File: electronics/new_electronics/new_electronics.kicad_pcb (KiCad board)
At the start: 2 copper layers, 165.1 x 101.6 mm, 48 parts, among them J1 PinHeader_1x03_P2.54mm_Vertic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, K1 Relay_SPDT_Omron-G5Q-1, K2 Relay_SPDT_Omron-G5Q-1, K3 Relay_SPDT_Omron-G5Q-1, K4 Relay_SPDT_Omron-G5Q-1, Q1 TO-92_Inline, Q2 TO-92_Inline, Q3 TO-92_Inline, Q4 TO-92_Inline, Q5 TO-92_Inline, Q6 TO-92_Inline, Q7 TO-92_Inline, Q8 TO-92_Inline, U1 metro_mini, U2 mpu6050

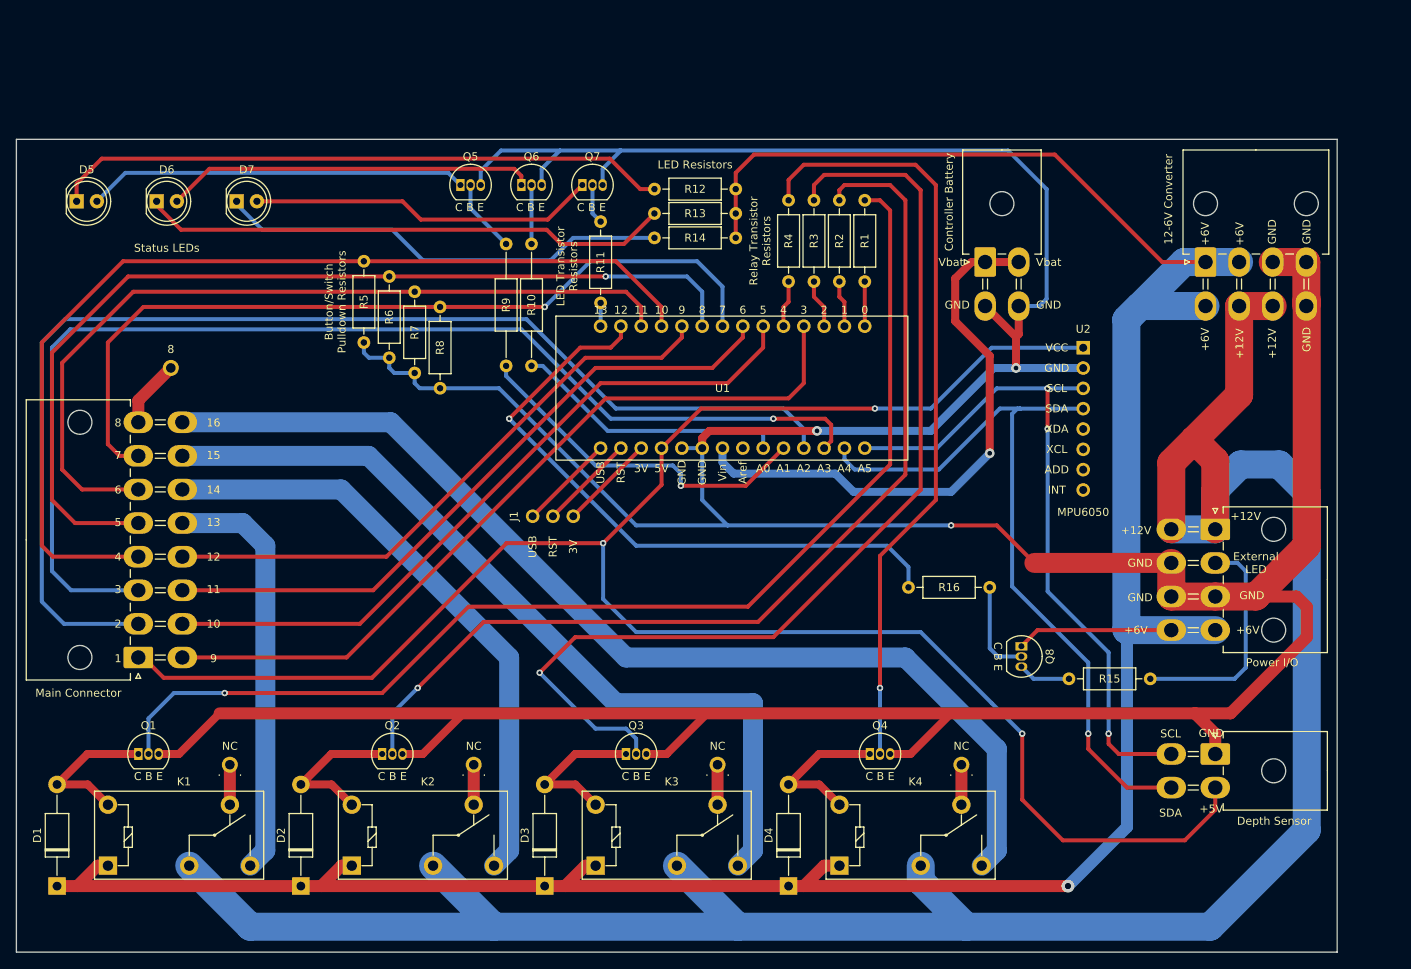
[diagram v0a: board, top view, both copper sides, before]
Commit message: modify pcb and schematic sheets for export for design report
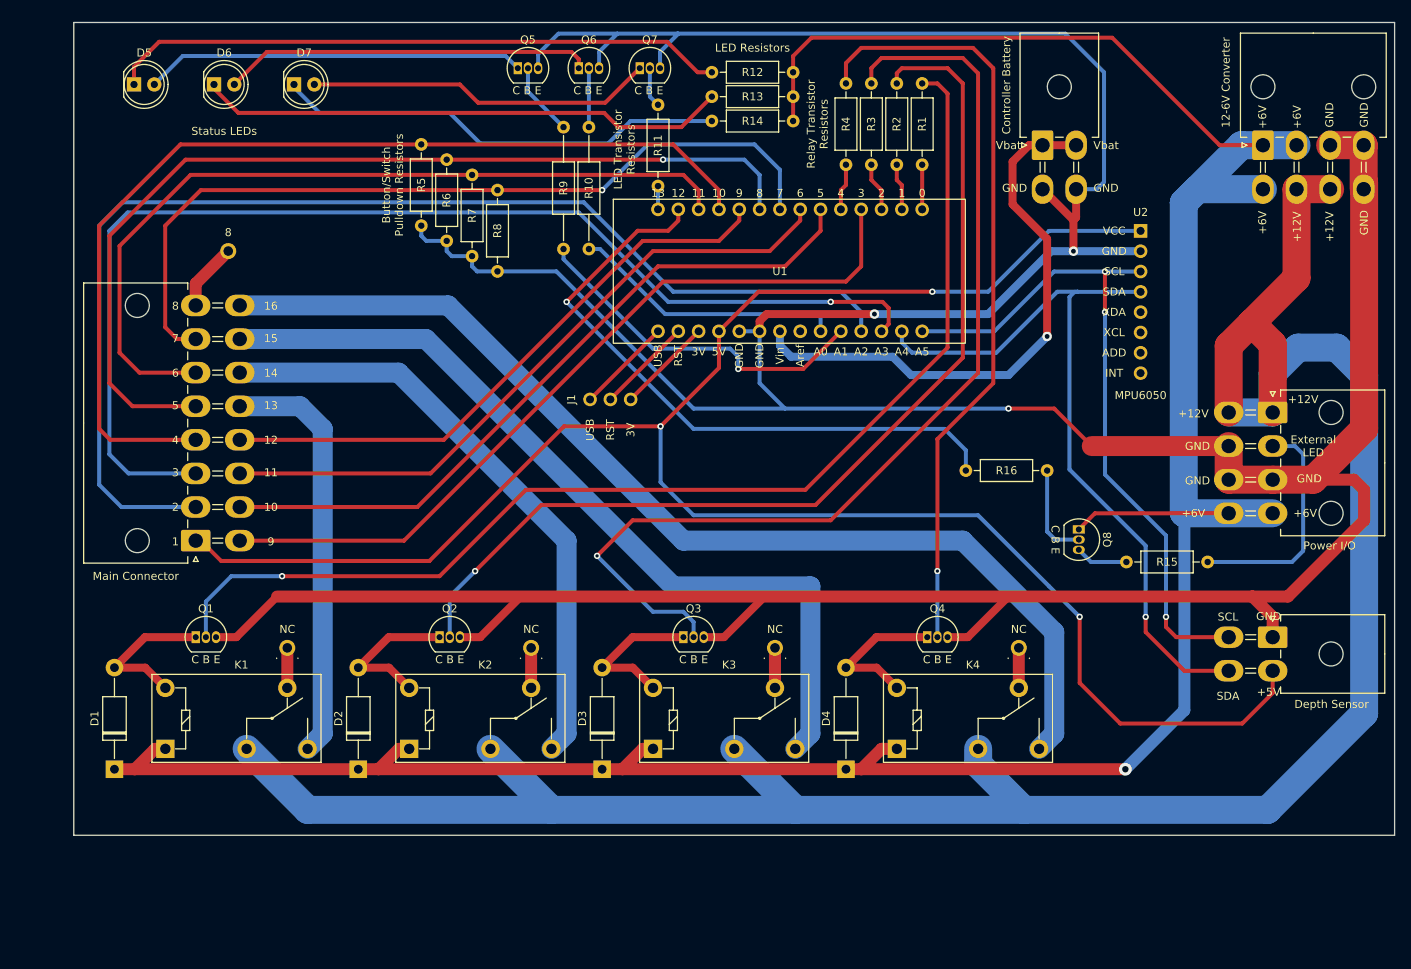
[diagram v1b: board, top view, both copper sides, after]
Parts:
- moved K1 16.3 mm to (66.9, 136.5)
- moved K2 16.3 mm to (97.4, 136.5)
- moved K3 16.3 mm to (127.8, 136.5)
- moved K4 16.3 mm to (158.3, 136.5)
- moved 8 16.3 mm to (74.7, 74.3)
- moved NC 16.3 mm to (82.1, 123.9)
- moved 12-6V Converter 16.3 mm to (204.1, 61.1)
- moved Controller Battery 16.3 mm to (176.5, 61.1)
- moved D5 16.3 mm to (63.0, 53.5)
- moved D6 16.3 mm to (73.0, 53.5)
- moved D7 16.3 mm to (83.0, 53.5)
- moved Main Connector 16.3 mm to (70.7, 110.5)
- moved NC 16.3 mm to (112.6, 123.9)
- moved NC 16.3 mm to (143.1, 123.9)
- moved NC 16.3 mm to (173.6, 123.9)
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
